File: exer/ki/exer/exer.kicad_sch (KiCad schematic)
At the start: 10 parts, among them U1 74HCT574, U2 74HCT574, U3 74HCT574, U4 74HCT574, U5 74HCT574, U6 74LS138, U7 74HCT574, U8 74HCT574, U9 74LS138

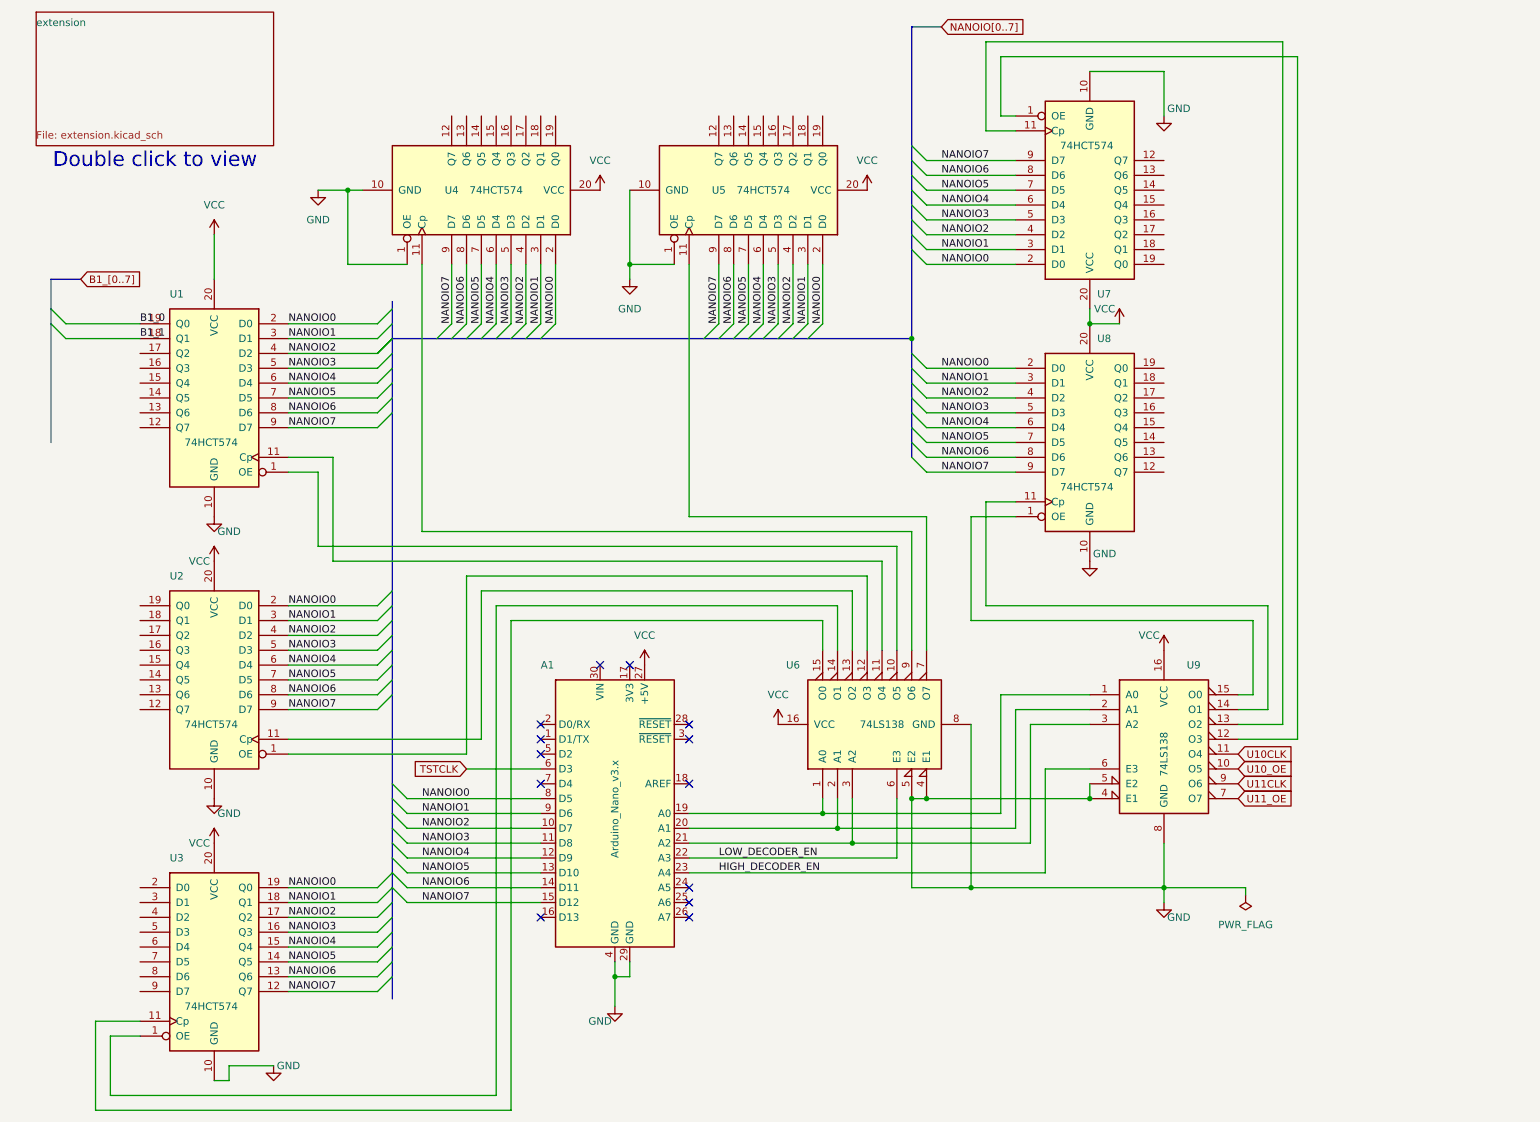
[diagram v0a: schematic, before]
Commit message: Ongoing development
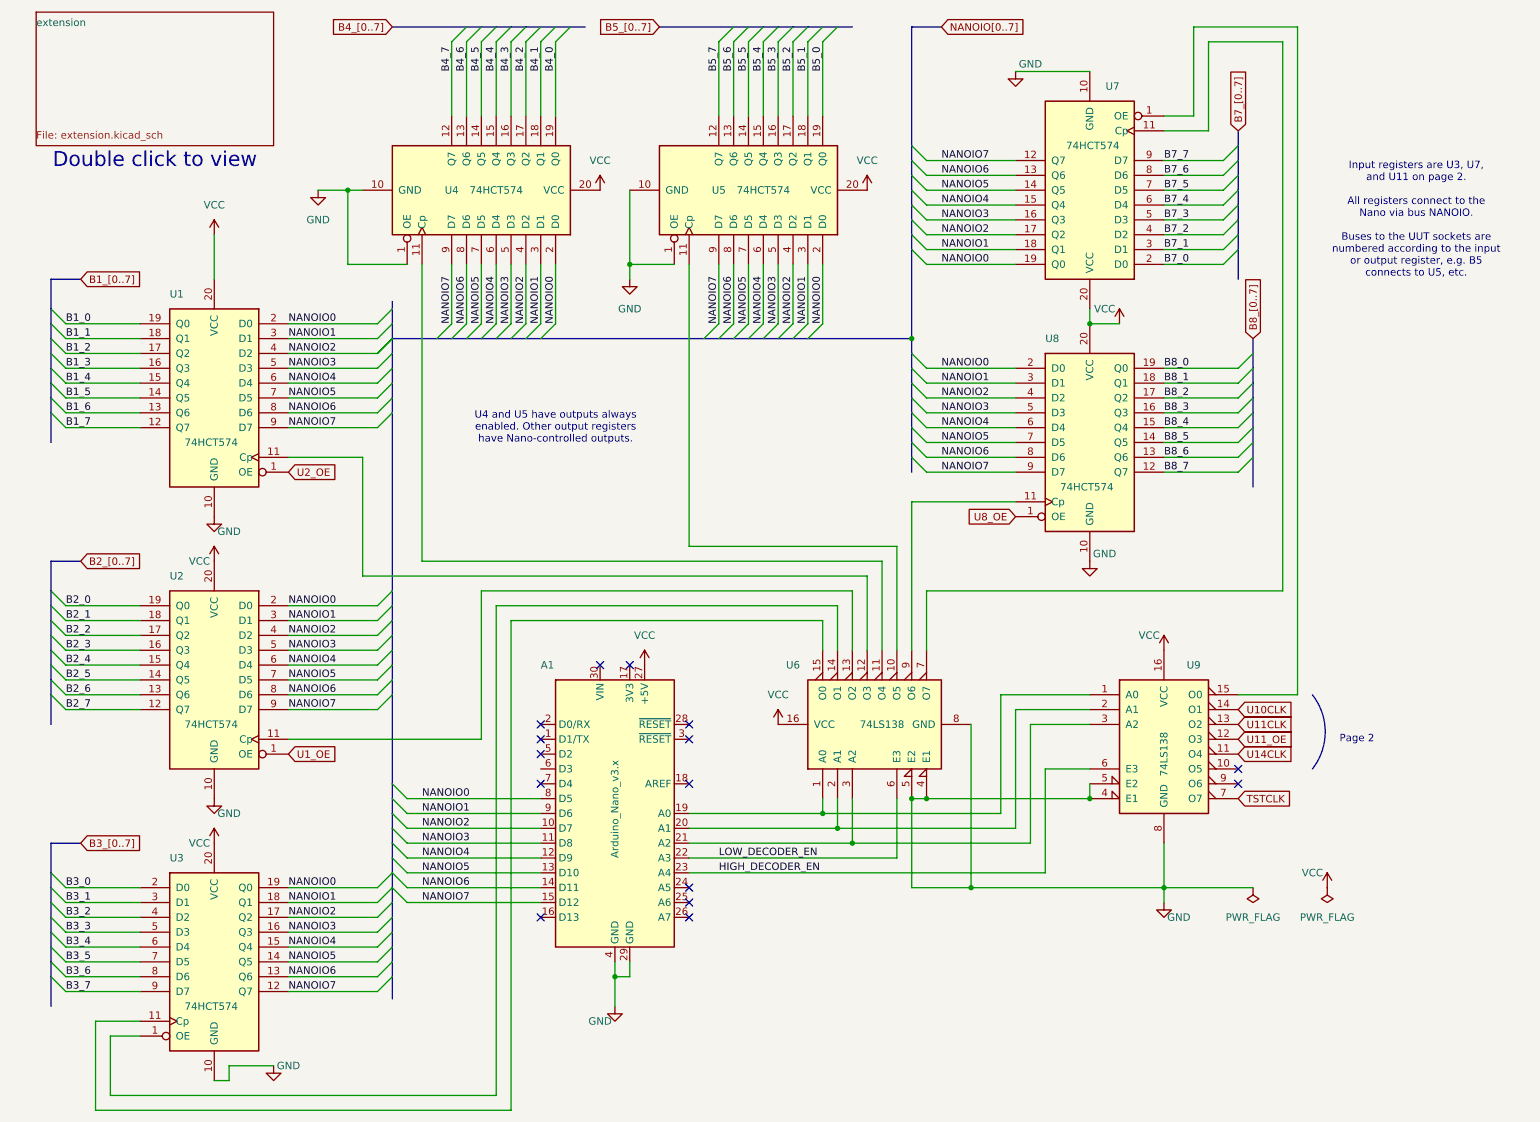
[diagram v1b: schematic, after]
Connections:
- net NANOIO0: now also U7.19 (Q0); no longer U7.2 (D0)
- net NANOIO1: now also U7.18 (Q1); no longer U7.3 (D1)
- net NANOIO2: now also U7.17 (Q2); no longer U7.4 (D2)
- net NANOIO3: now also U7.16 (Q3); no longer U7.5 (D3)
- net NANOIO4: now also U7.15 (Q4); no longer U7.6 (D4)
- net NANOIO5: now also U7.14 (Q5); no longer U7.7 (D5)
- net NANOIO6: now also U7.13 (Q6); no longer U7.8 (D6)
- net NANOIO7: now also U7.12 (Q7); no longer U7.9 (D7)
- net TSTCLK: now also U9.7 (O7); no longer A1.6 (D3)
- net U10CLK: now also U9.14 (O1); no longer U9.11 (O4)
- net U11CLK: now also U9.13 (O2); no longer U9.9 (O6)
- net U11_OE: now also U9.12 (O3); no longer U9.7 (O7)
- net at U7.1 (OE): now also U9.15 (O0); no longer U9.12 (O3)
- net at U7.11 (Cp): now also U6.7 (O7); no longer U9.13 (O2)
- net at U8.11 (Cp): now also U6.9 (O6); no longer U9.14 (O1)
- net U8_OE: now reaches U8.1 (OE)
- net U8_OE: no longer U9.15 (O0)
- net at U4.11 (Cp): now also U6.11 (O4); no longer U6.9 (O6)
- net B4_7: now reaches U4.12 (Q7)
- net B4_6: now reaches U4.13 (Q6)
- net B4_5: now reaches U4.14 (Q5)
- net B4_4: now reaches U4.15 (Q4)
- net B4_3: now reaches U4.16 (Q3)
- net B4_2: now reaches U4.17 (Q2)
- net B4_1: now reaches U4.18 (Q1)
- net B4_0: now reaches U4.19 (Q0)
- net B3_0: now reaches U3.2 (D0)
- net B3_1: now reaches U3.3 (D1)
- net B3_2: now reaches U3.4 (D2)
- net B3_3: now reaches U3.5 (D3)
- net B3_4: now reaches U3.6 (D4)
- net B3_5: now reaches U3.7 (D5)
- net B3_6: now reaches U3.8 (D6)
- net B3_7: now reaches U3.9 (D7)
- net at U6.12 (O3): now also U1.11 (Cp); no longer U2.1 (OE)
- net B2_7: now reaches U2.12 (Q7)
- net B2_6: now reaches U2.13 (Q6)
- net B2_5: now reaches U2.14 (Q5)
- net B2_4: now reaches U2.15 (Q4)
- net B2_3: now reaches U2.16 (Q3)
- net B2_2: now reaches U2.17 (Q2)
- net B2_1: now reaches U2.18 (Q1)
- net B2_0: now reaches U2.19 (Q0)
- net at U6.10 (O5): now also U5.11 (Cp); no longer U1.1 (OE)
- net B1_7: now reaches U1.12 (Q7)
- net B1_6: now reaches U1.13 (Q6)
- net B1_5: now reaches U1.14 (Q5)
- net B1_4: now reaches U1.15 (Q4)
- net B1_3: now reaches U1.16 (Q3)
- net B1_2: now reaches U1.17 (Q2)
- net B5_7: now reaches U5.12 (Q7)
- net B5_6: now reaches U5.13 (Q6)
- net B5_5: now reaches U5.14 (Q5)
- net B5_4: now reaches U5.15 (Q4)
- net B5_3: now reaches U5.16 (Q3)
- net B5_2: now reaches U5.17 (Q2)
- net B5_1: now reaches U5.18 (Q1)
- net B5_0: now reaches U5.19 (Q0)
- net B8_7: now reaches U8.12 (Q7)
- net B8_6: now reaches U8.13 (Q6)
- net B8_5: now reaches U8.14 (Q5)
- net B8_4: now reaches U8.15 (Q4)
- net B8_3: now reaches U8.16 (Q3)
- net B8_2: now reaches U8.17 (Q2)
- net B8_1: now reaches U8.18 (Q1)
- net B8_0: now reaches U8.19 (Q0)
- net U10_OE: no longer names the net of U9.10 (O5)
- new net B7_0: U7.2 (D0)
- new net B7_1: U7.3 (D1)
- new net B7_2: U7.4 (D2)
- new net B7_3: U7.5 (D3)
- new net B7_4: U7.6 (D4)
- new net B7_5: U7.7 (D5)
- new net B7_6: U7.8 (D6)
- new net B7_7: U7.9 (D7)
- new net U14CLK: U9.11 (O4)
- new net U1_OE: U2.1 (OE)
- new net U2_OE: U1.1 (OE)
- no-connect marks 13 -> 15
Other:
- note added: "Input registers are U3, U7, and U11 on page 2. All registers connect to the Nano via bus NANOIO. Buses to the UUT sockets are numbered according to the input or output register, e.g. B5 connects to U5, etc."
- note added: "Page 2"
- note added: "U4 and U5 have outputs always enabled. Other output registers have Nano-controlled outputs."
- moved on the sheet: U7

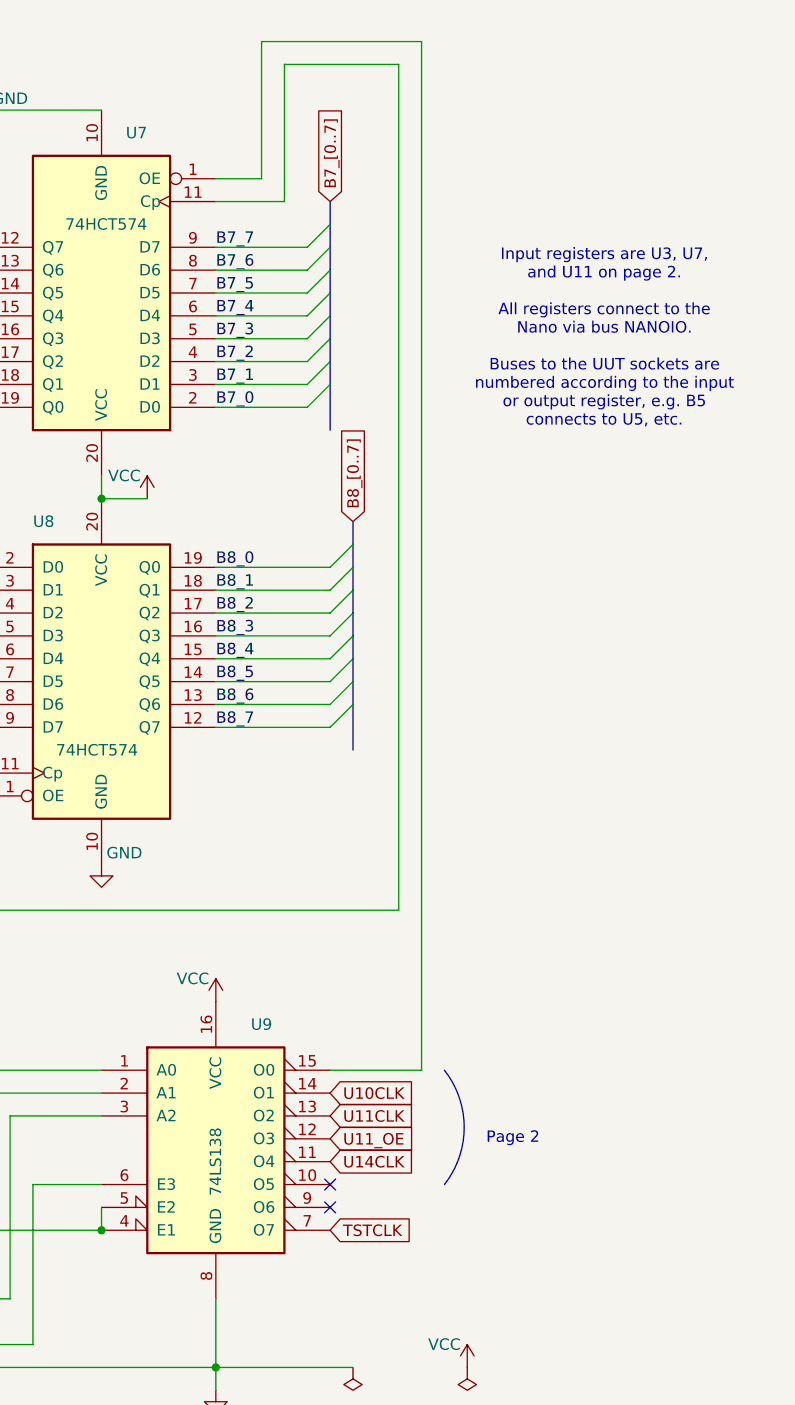
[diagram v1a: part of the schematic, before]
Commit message: Ongoing development of chip exerciser
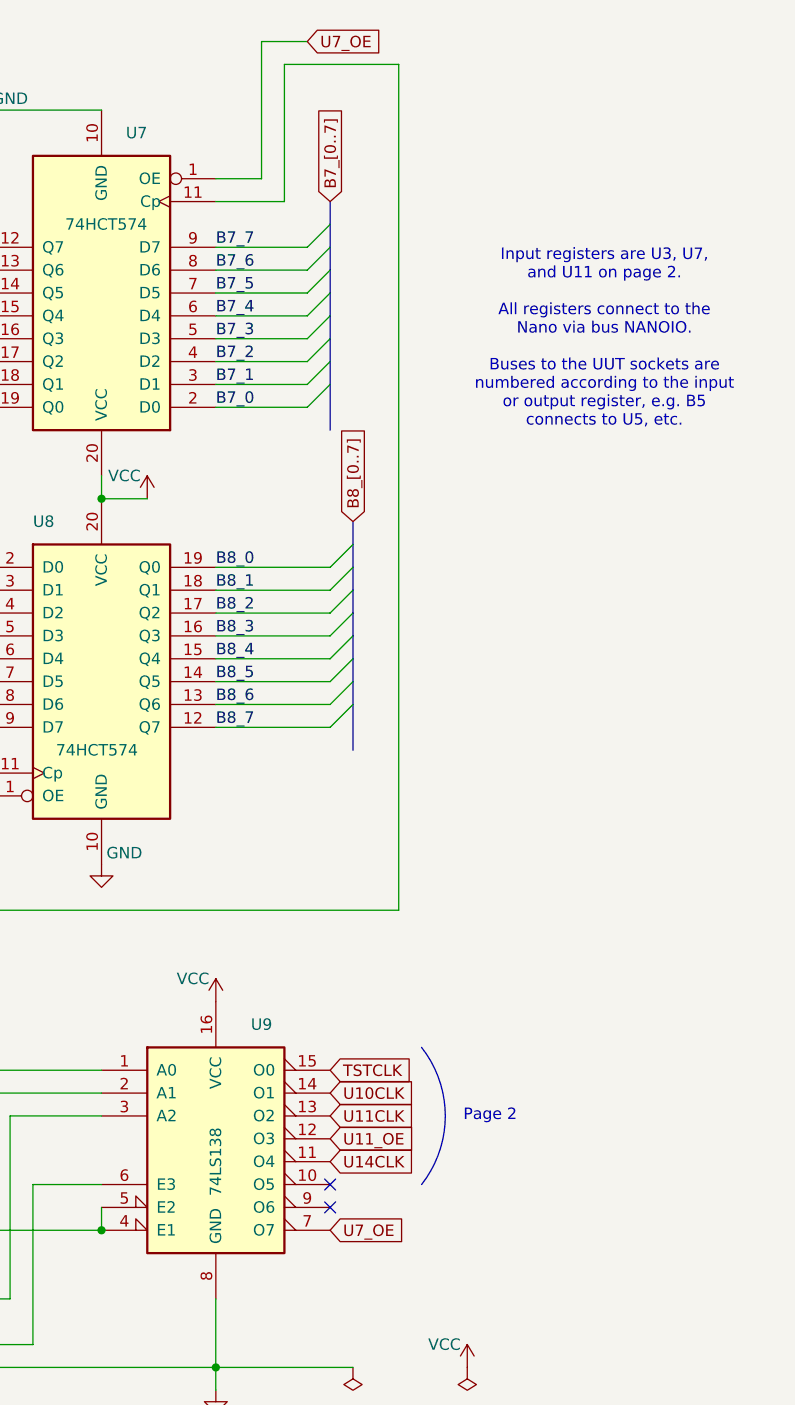
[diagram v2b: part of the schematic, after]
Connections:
- net TSTCLK: now also U9.15 (O0); no longer U9.7 (O7)
- net U7_OE: now reaches U7.1 (OE)
- net U7_OE: now also U9.7 (O7); no longer U9.15 (O0)
